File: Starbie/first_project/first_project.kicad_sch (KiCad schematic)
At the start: 7 parts, among them J1 Conn_01x04_Pin, J2 Conn_01x08_Pin, SW1 SW_Push, SW2 SW_Push, U1 DHT11, U2 XIAO-ESP32-C3-SMD

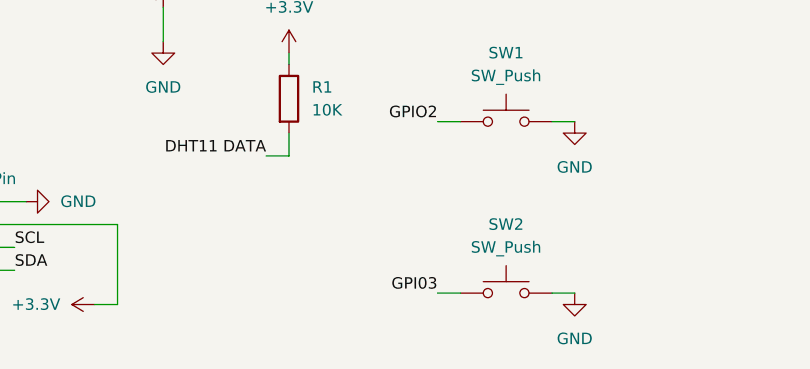
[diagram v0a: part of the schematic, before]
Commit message: ChromeOS Migration
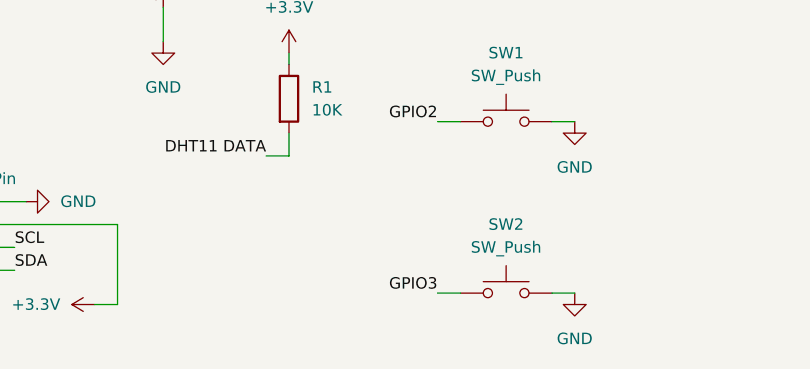
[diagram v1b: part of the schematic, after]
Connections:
- net GPI03 is gone; now on net GPIO3: SW2.1
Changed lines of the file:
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@@
 		)
 	)
-	(label "GPI03"
+	(label "GPIO3"
 		(at 86.36 119.38 180)
 		(effects
